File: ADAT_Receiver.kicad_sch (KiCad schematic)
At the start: 21 parts, among them J1 USB_C_Receptacle_PowerOnly_6P, J2 PLR135-T, J3 Conn_01x07_Pin, J4 Conn_01x05_Pin, J5 PLx13xT, SW1 SW_DIP_x03, U1 V1402

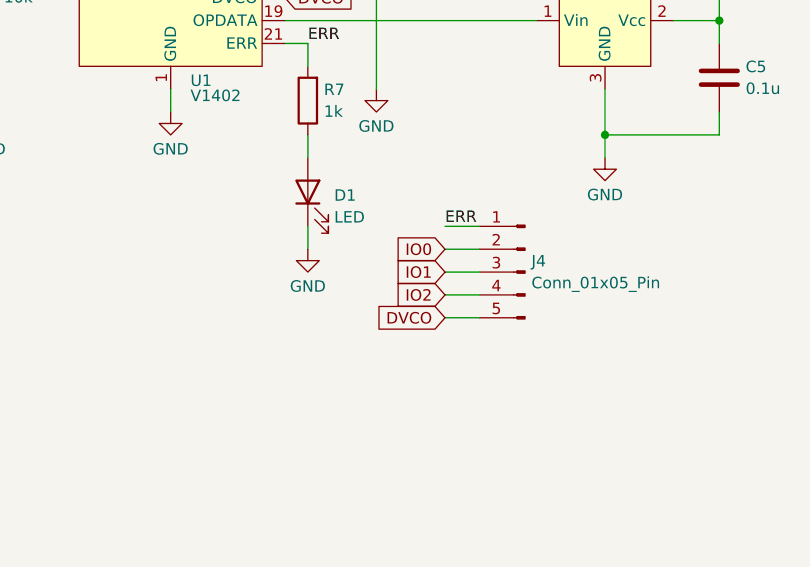
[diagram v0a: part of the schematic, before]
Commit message: First order
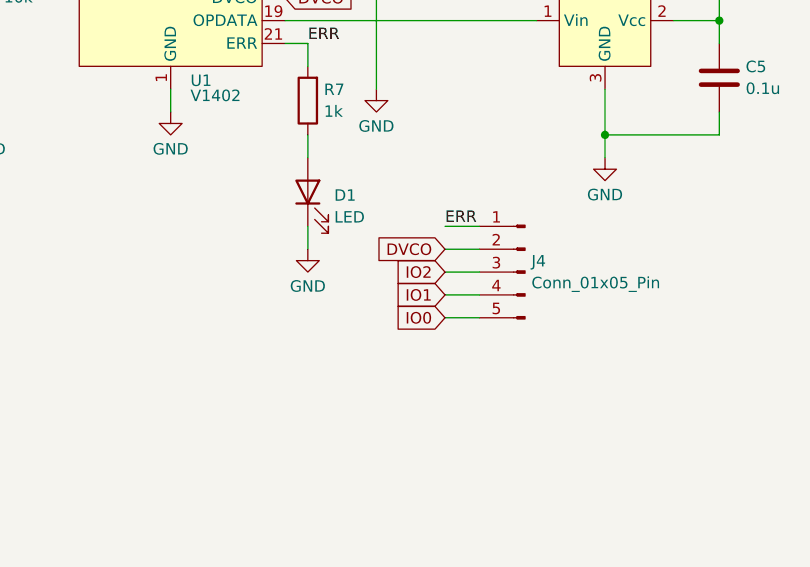
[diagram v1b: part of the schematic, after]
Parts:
- SW1: footprint Button_Switch_SMD:SW_DIP_SPSTx03_Slide_6.7x9.18mm_W6.73mm_P2.54mm_LowProfile_JPin -> Button_Switch_SMD:SW_DIP_SPSTx03_Slide_6.7x9.18mm_W8.61mm_P2.54mm_LowProfile
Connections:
- net DVCO: now also J4.2 (Pin_2); no longer J4.5 (Pin_5)
- net IO0: now also J4.5 (Pin_5); no longer J4.2 (Pin_2)
- net IO1: now also J4.4 (Pin_4); no longer J4.3 (Pin_3)
- net IO2: now also J4.3 (Pin_3); no longer J4.4 (Pin_4)
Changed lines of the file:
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@@
 	(global_label "DVCO"
 		(shape input)
+		(at 167.64 111.76 180)
+		(fields_autoplaced yes)
+		(effects
+			(font
+				(size 1.27 1.27)
+			)
+			(justify right)
+		)
+		(property "Intersheetrefs" "${INTERSHEET_REFS}"
+			(at 159.6957 111.76 0)
+			(effects
+				(font
+					(size 1.27 1.27)
+				)
+				(justify right)
+				(hide yes)
+			)
+		)
+	)
+	(global_label "IO0"
+		(shape input)
 		(at 167.64 119.38 180)
 		(fields_autoplaced yes)
@@
 		)
 		(property "Intersheetrefs" "${INTERSHEET_REFS}"
-			(at 159.6957 119.38 0)
+			(at 161.51 119.38 0)
+			(effects
+				(font
+					(size 1.27 1.27)
+				)
+				(justify right)
+				(hide yes)
+			)
+		)
+	)
+	(global_label "DVCO"
+		(shape input)
+		(at 149.86 83.82 0)
+		(fields_autoplaced yes)
+		(effects
+			(font
+				(size 1.27 1.27)
+			)
+			(justify left)
+		)
+		(property "Intersheetrefs" "${INTERSHEET_REFS}"
+			(at 157.8043 83.82 0)
+			(effects
+				(font
+					(size 1.27 1.27)
+				)
+				(justify left)
+				(hide yes)
+			)
+		)
+	)
+	(global_label "IO2"
+		(shape input)
+		(at 167.64 114.3 180)
+		(fields_autoplaced yes)
+		(effects
+			(font
+				(size 1.27 1.27)
+			)
+			(justify right)
+		)
+		(property "Intersheetrefs" "${INTERSHEET_REFS}"
+			(at 161.51 114.3 0)
 			(effects
 				(font
@@
 	(global_label "IO0"
 		(shape input)
-		(at 167.64 111.76 180)
+		(at 149.86 73.66 0)
+		(fields_autoplaced yes)
+		(effects
+			(font
+				(size 1.27 1.27)
+			)
+			(justify left)
+		)
+		(property "Intersheetrefs" "${INTERSHEET_REFS}"
+			(at 155.99 73.66 0)
+			(effects
+				(font
+					(size 1.27 1.27)
+				)
+				(justify left)
+				(hide yes)
+			)
+		)
+	)
+	(global_label "IO1"
+		(shape input)
+		(at 167.64 116.84 180)
 		(fields_autoplaced yes)
 		(effects
@@
 		)
 		(property "Intersheetrefs" "${INTERSHEET_REFS}"
-			(at 161.51 111.76 0)
-			(effects
-				(font
-					(size 1.27 1.27)
-				)
-				(justify right)
-				(hide yes)
-			)
-		)
-	)
-	(global_label "DVCO"
-		(shape input)
-		(at 149.86 83.82 0)
-		(fields_autoplaced yes)
-		(effects
-			(font
-				(size 1.27 1.27)
-			)
-			(justify left)
-		)
-		(property "Intersheetrefs" "${INTERSHEET_REFS}"
-			(at 157.8043 83.82 0)
-			(effects
-				(font
-					(size 1.27 1.27)
-				)
-				(justify left)
-				(hide yes)
-			)
-		)
-	)
-	(global_label "IO2"
-		(shape input)
-		(at 167.64 116.84 180)
-		(fields_autoplaced yes)
-		(effects
-			(font
-				(size 1.27 1.27)
-			)
-			(justify right)
-		)
-		(property "Intersheetrefs" "${INTERSHEET_REFS}"
 			(at 161.51 116.84 0)
-			(effects
-				(font
-					(size 1.27 1.27)
-				)
-				(justify right)
-				(hide yes)
-			)
-		)
-	)
-	(global_label "IO0"
-		(shape input)
-		(at 149.86 73.66 0)
-		(fields_autoplaced yes)
-		(effects
-			(font
-				(size 1.27 1.27)
-			)
-			(justify left)
-		)
-		(property "Intersheetrefs" "${INTERSHEET_REFS}"
-			(at 155.99 73.66 0)
-			(effects
-				(font
-					(size 1.27 1.27)
-				)
-				(justify left)
-				(hide yes)
-			)
-		)
-	)
-	(global_label "IO1"
-		(shape input)
-		(at 167.64 114.3 180)
-		(fields_autoplaced yes)
-		(effects
-			(font
-				(size 1.27 1.27)
-			)
-			(justify right)
-		)
-		(property "Intersheetrefs" "${INTERSHEET_REFS}"
-			(at 161.51 114.3 0)
 			(effects
 				(font
@@
 			)
 		)
-		(property "Footprint" "Button_Switch_SMD:SW_DIP_SPSTx03_Slide_6.7x9.18mm_W6.73mm_P2.54mm_LowProfile_JPin"
+		(property "Footprint" "Button_Switch_SMD:SW_DIP_SPSTx03_Slide_6.7x9.18mm_W8.61mm_P2.54mm_LowProfile"
 			(at 73.66 38.1 0)
 			(effects
